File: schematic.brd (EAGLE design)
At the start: 166.3 x 125.4 mm, 31 parts, among them IC1 ATMEGA32L-8AU, J1 POWER_JACKPTH_BREAD

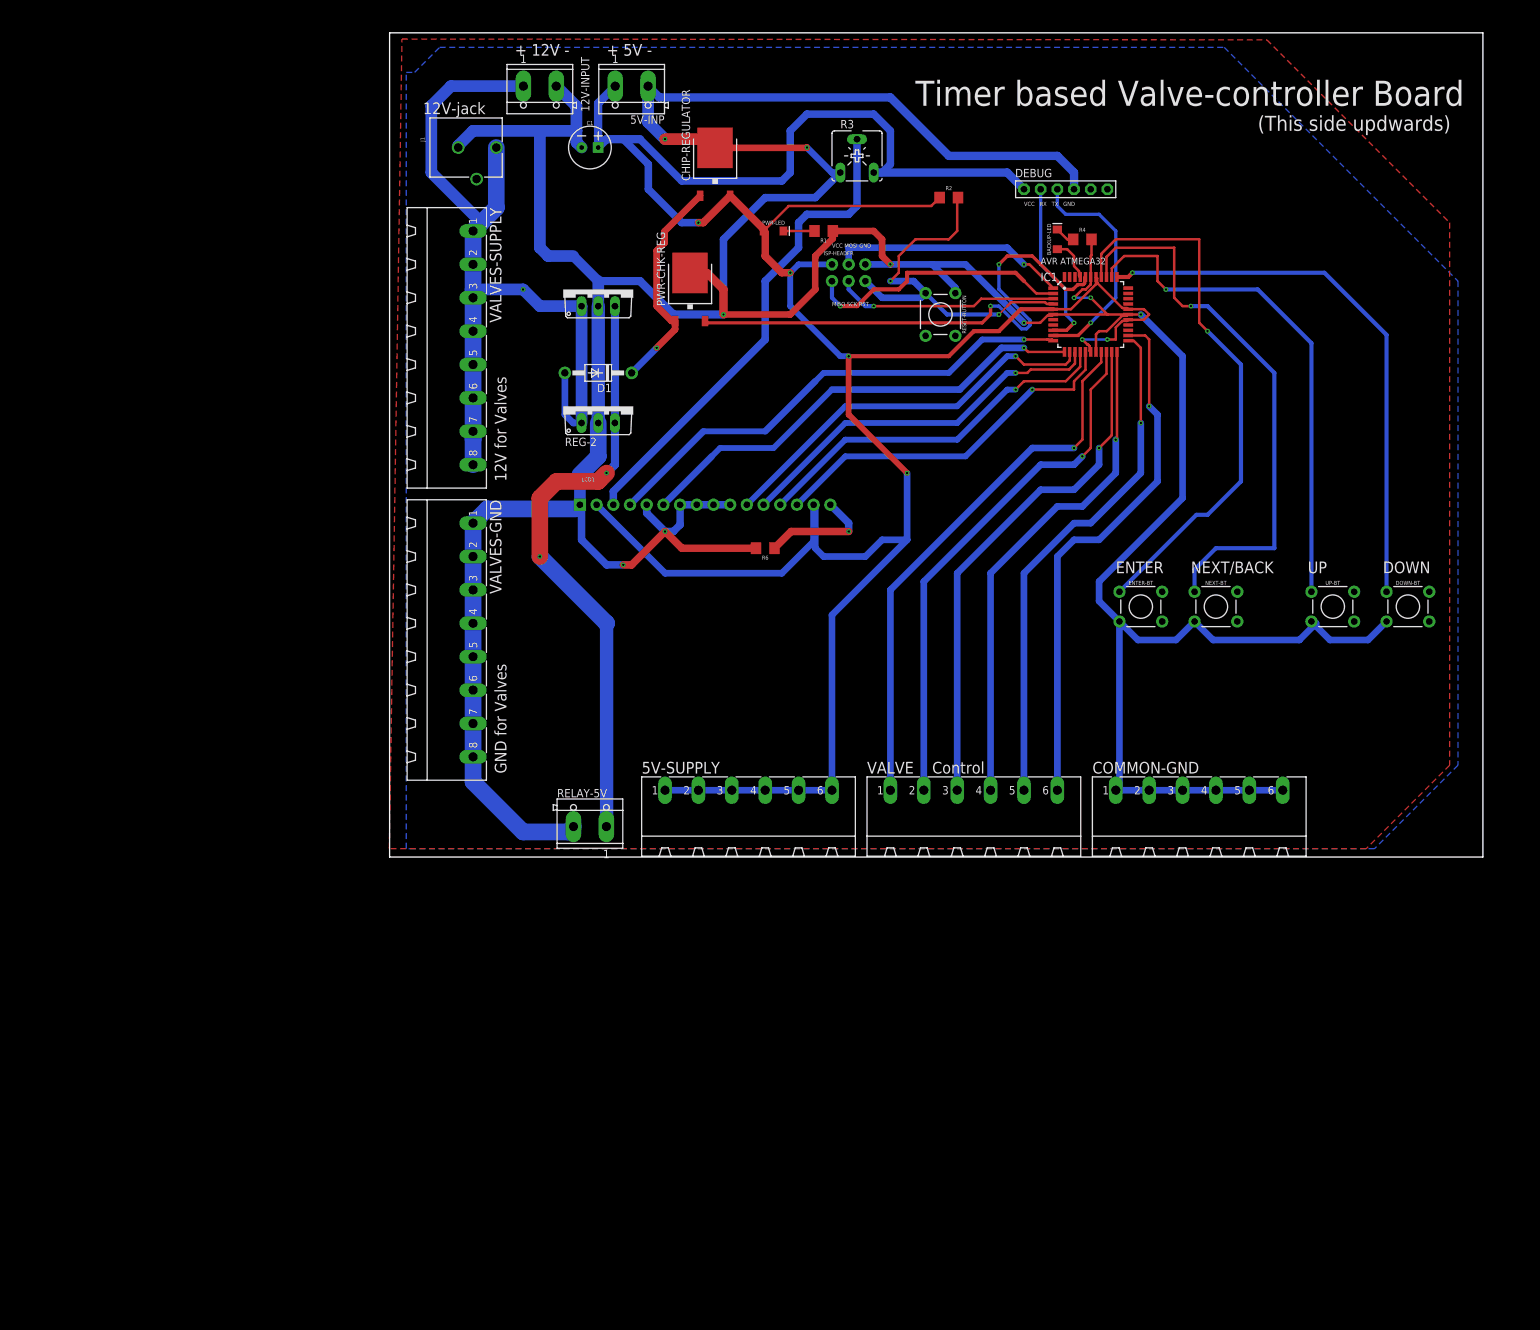
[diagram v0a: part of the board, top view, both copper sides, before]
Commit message: test commit by me
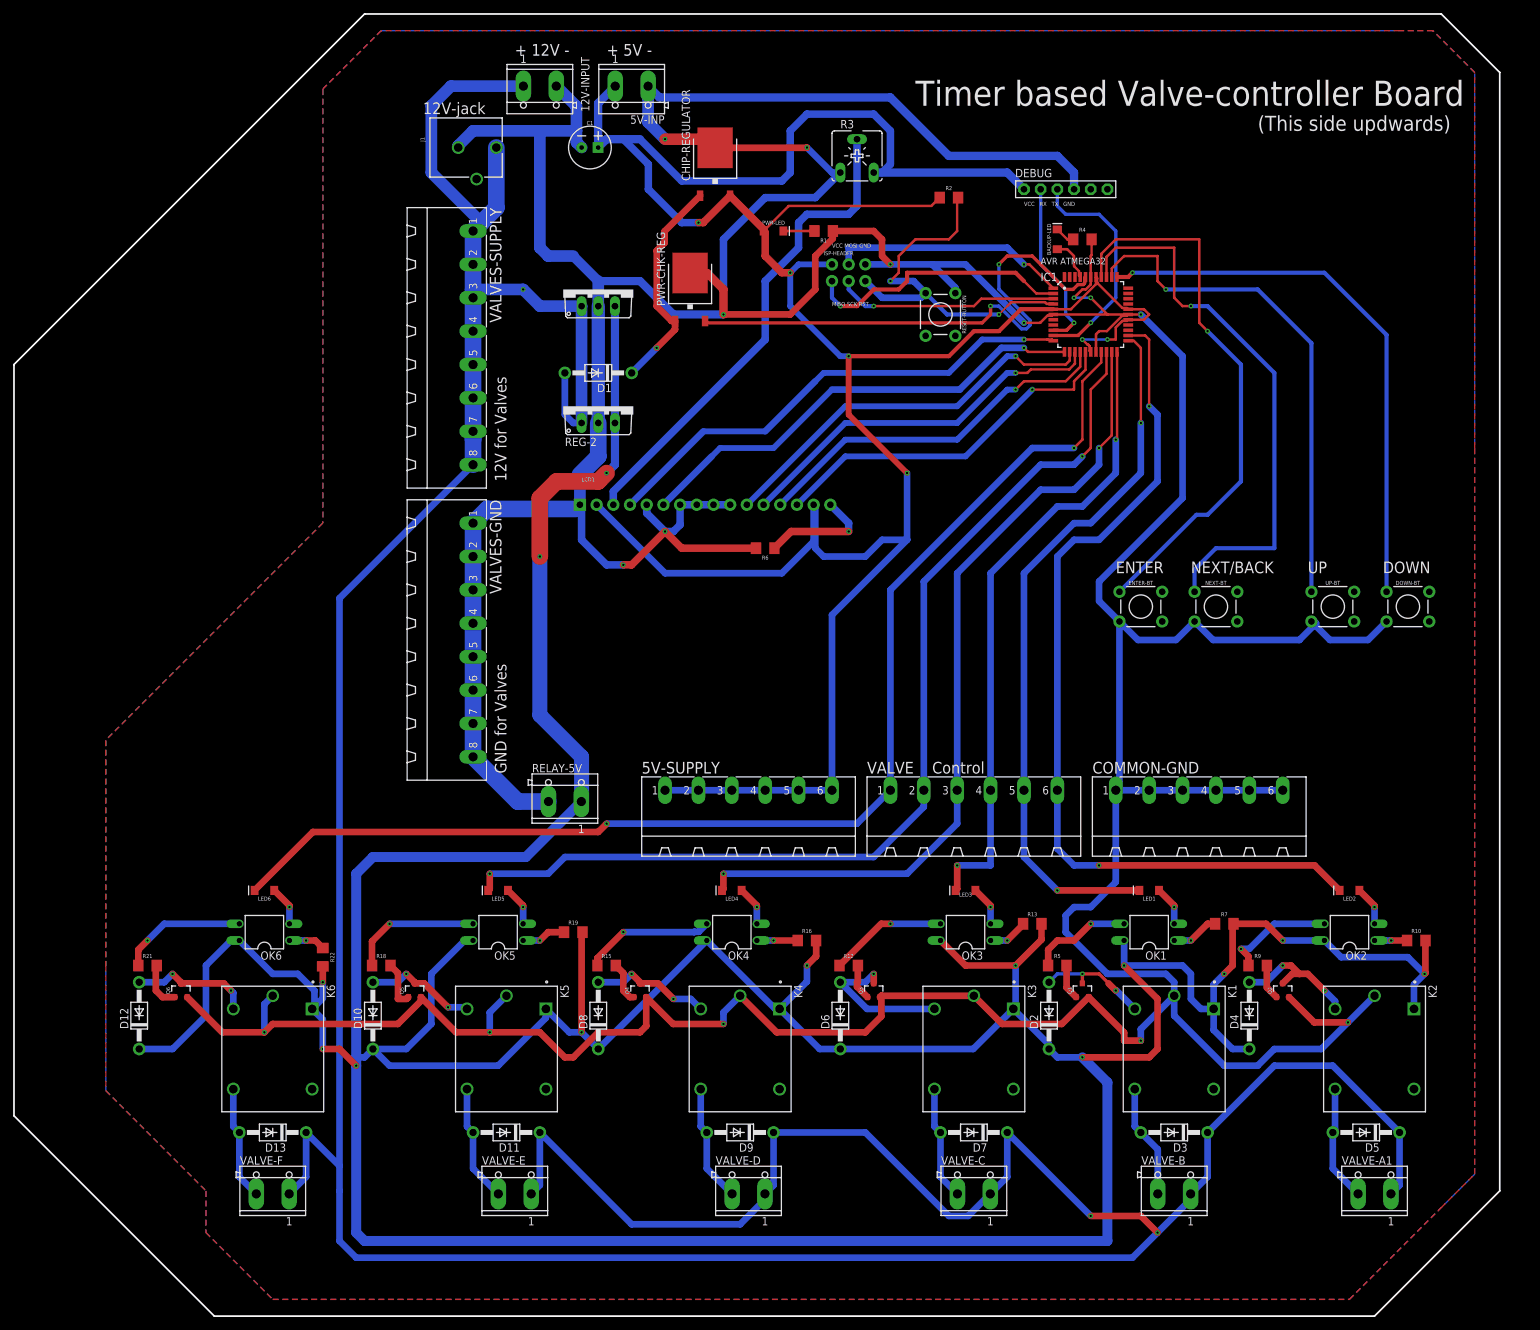
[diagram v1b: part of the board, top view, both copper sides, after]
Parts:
- added D10, D11, D12, D13, D2, D3, D4, D5, D6, D7, D8, D9: 1N4004, adafruit:DO41-10
- added K1, K2, K3, K4, K5, K6: SRD-05VDC-SL-C, SRD-05VDC-SL-C:RELAY_SRD-05VDC-SL-C
- added LED1, LED2, LED3, LED4, LED5, LED6: (no value), SparkFun-Retired:LED-1206
- added OK1, OK2, OK3, OK4, OK5, OK6: PC817, optocoupler:DIL04
- added Q1, Q2, Q3, Q4, Q5, Q6: 500mA/300V, SparkFun-DiscreteSemi:SOT23-3
- added R10, R12, R13, R15, R16, R18, R19, R21, R22, R5, R7, R9: (no value), SparkFun-Resistors:1206
- added VALVE-A1, VALVE-B, VALVE-C, VALVE-D, VALVE-E, VALVE-F: CON_TERMINAL_BLOCK_02-5MM, dp_devices:TERMINAL_BLOCK_2P_5
- BACKUP-LED: value (none) -> red
- R3: value (none) -> 10k
- moved RELAY-5V 5.39 mm to (24.1, -3.81)
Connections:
- new net N$10: Q1.1, R5.2
- new net N$11: OK2.1, R10.1
- new net N$12: D3.A, K1.NO, VALVE-B.2
- new net N$13: LED2.A, OK2.2
- new net N$14: OK2.3, R9.1
- new net N$15: Q2.1, R9.2
- new net N$16: D4.A, K2.A2, Q2.3
- new net N$17: D5.A, K2.NO, VALVE-A1.2
- new net N$18: OK3.1, R13.1
- new net N$19: LED3.A, OK3.2
- new net N$20: OK3.3, R12.1
- new net N$21: Q3.1, R12.2
- new net N$22: D6.A, K3.A2, Q3.3
- new net N$23: D7.A, K3.NO, VALVE-C.2
- new net N$24: OK4.1, R16.1
- new net N$25: LED4.A, OK4.2
- new net N$26: OK4.3, R15.1
- new net N$27: Q4.1, R15.2
- new net N$28: D8.A, K4.A2, Q4.3
- new net N$29: D9.A, K4.NO, VALVE-D.2
- new net N$3: OK1.1, R7.1
- new net N$30: OK5.1, R19.1
- new net N$31: LED5.A, OK5.2
- new net N$32: OK5.3, R18.1
- new net N$33: Q5.1, R18.2
- new net N$34: D10.A, K5.A2, Q5.3
- new net N$35: D11.A, K5.NO, VALVE-E.2
- new net N$36: OK6.1, R22.1
- new net N$37: LED6.A, OK6.2
- new net N$38: OK6.3, R21.1
- new net N$39: Q6.1, R21.2
- new net N$40: D12.A, K6.A2, Q6.3
- new net N$41: D13.A, K6.NO, VALVE-F.2
- new net N$7: LED1.A, OK1.2
- new net N$8: OK1.3, R5.1
- new net N$9: D2.A, K1.A2, Q1.3
- net 12VDC: now also D11.C, D13.C, D3.C, D5.C, D7.C, D9.C, VALVE-A1.1, VALVE-B.1, VALVE-C.1, VALVE-D.1, VALVE-E.1, VALVE-F.1
- net 5V-RELAY: now also D10.C, D12.C, D2.C, D4.C, D6.C, D8.C, K1.A1, K2.A1, K3.A1, K4.A1, K5.A1, K6.A1, OK1.4, OK2.4, OK3.4, OK4.4, OK5.4, OK6.4, R10.2, R13.2, R16.2, R19.2, R22.2, R7.2
- net GND: now also K1.COM, K2.COM, K3.COM, K4.COM, K5.COM, K6.COM, Q1.2, Q2.2, Q3.2, Q4.2, Q5.2, Q6.2
- net VAL-A: now also LED2.C
- net VAL-B: now also LED1.C
- net VAL-C: now also LED3.C
- net VAL-D: now also LED4.C
- net VAL-E: now also LED5.C
- net VAL-F: now also LED6.C
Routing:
- net 5V-RELAY: track 92.8 -> 725.3 mm, vias 2 -> 13
- net 12VDC: track 135.7 -> 614.3 mm, vias 1 -> 3
- net GND: track 690.5 -> 981.6 mm, vias 10 -> 15
- net VAL-F: track 83.7 -> 186.8 mm, vias 1 -> 2
- net VAL-E: track 81.2 -> 156.6 mm, vias 1 -> 2
- net VAL-A: track 81.1 -> 135.6 mm, vias 1 -> 2
- net VAL-D: track 79.4 -> 125.8 mm, vias 1 -> 2
- net VAL-B: track 78.5 -> 108.3 mm, vias 1 -> 2
- net N$22: track 0.00 -> 23.0 mm, vias 0 -> 1
- net N$16: track 0.00 -> 20.7 mm, vias 0 -> 2
- net VAL-C: track 76.9 -> 97.3 mm, vias 1 -> 2
- net N$32: track 0.00 -> 20.2 mm, vias 0 -> 1
- net N$26: track 0.00 -> 19.9 mm, vias 0 -> 1
- net N$38: track 0.00 -> 19.4 mm, vias 0 -> 1
- net N$40: track 0.00 -> 18.6 mm, vias 0 -> 2
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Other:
- board size 166.3 x 125.4 mm -> 226.1 x 198.1 mm
